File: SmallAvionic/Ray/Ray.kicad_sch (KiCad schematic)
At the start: 12 parts, among them U1 STM32F103C8Tx, U2 BMI088

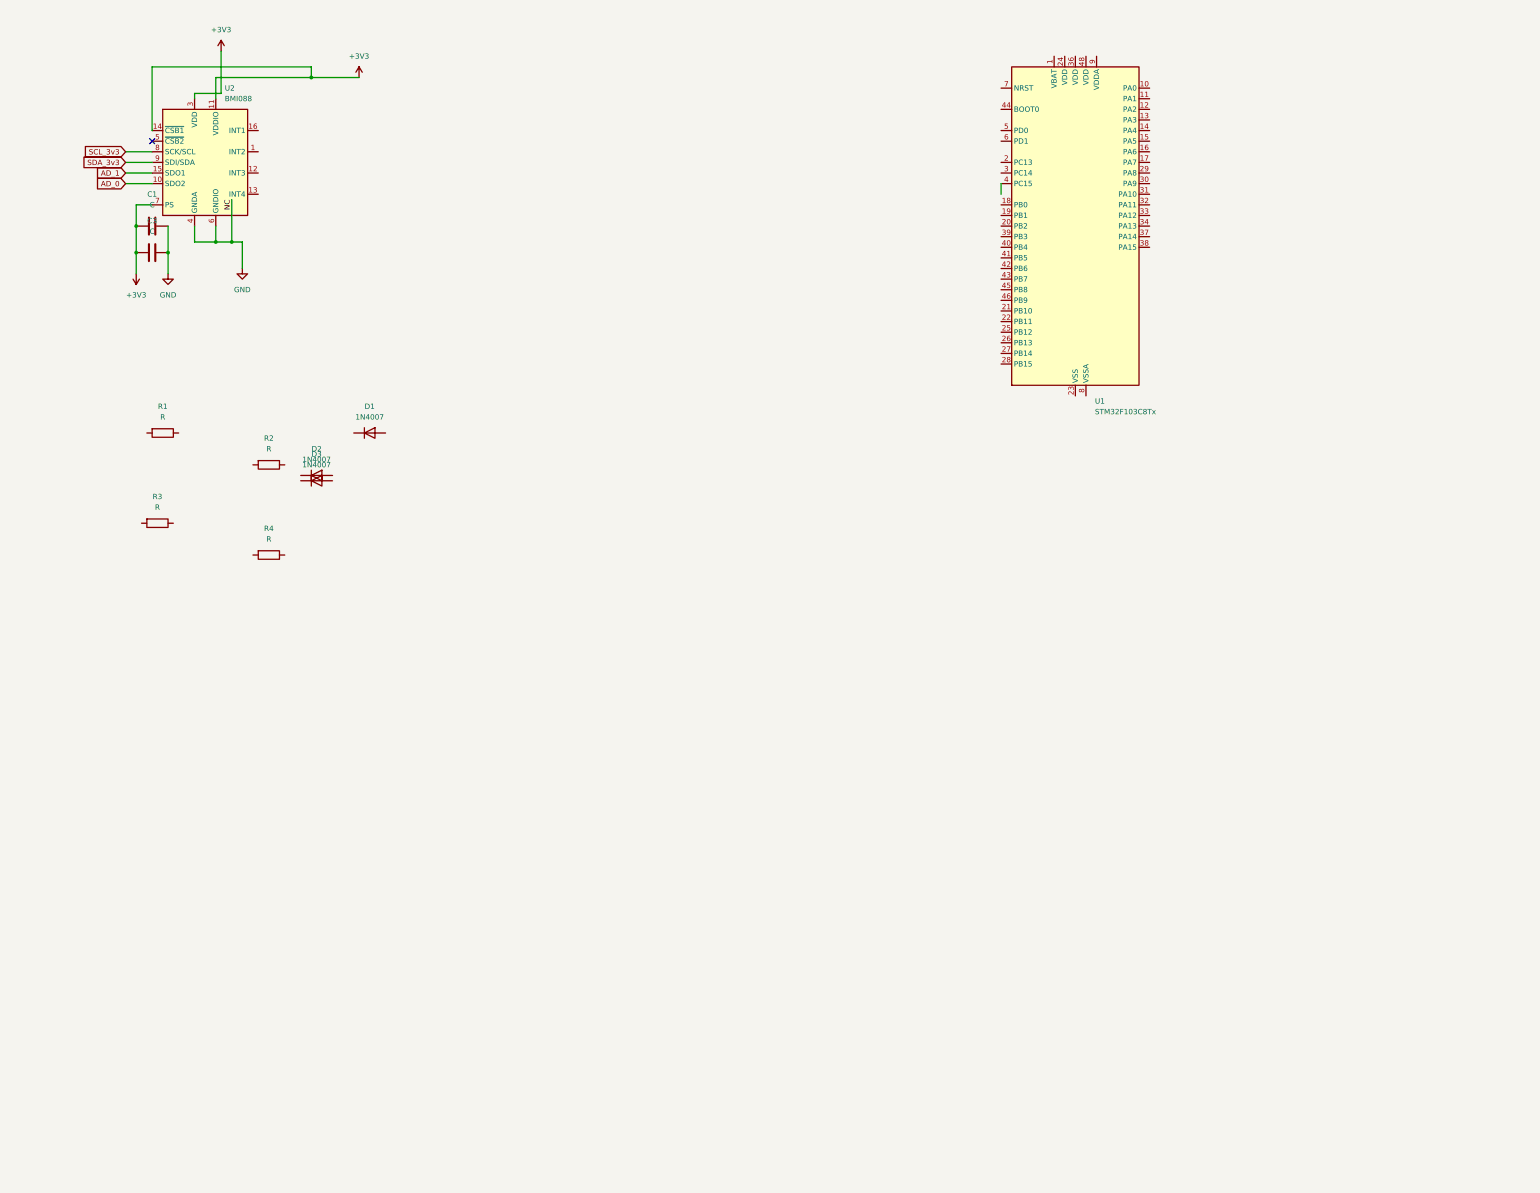
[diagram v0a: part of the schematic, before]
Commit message: Ray finish IMU,BMP, Madnetometer. But just whatever3 7 21 copy from internet
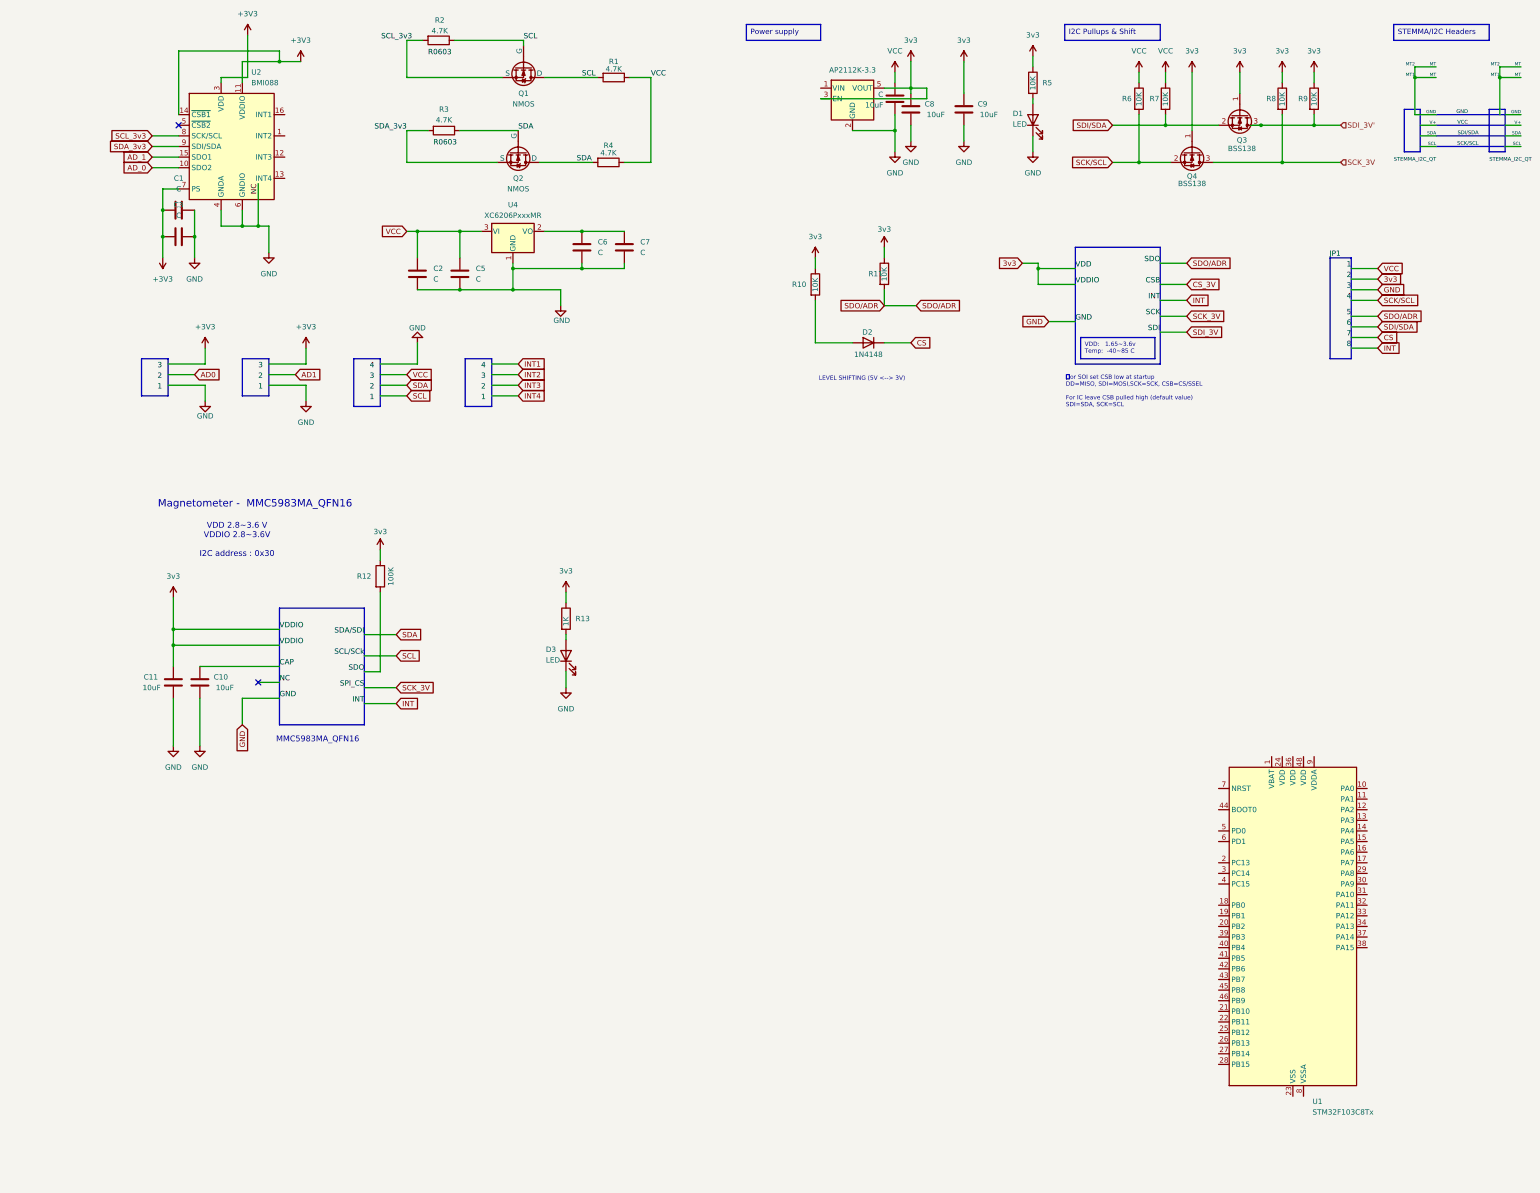
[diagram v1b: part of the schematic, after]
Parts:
- removed D1, D2, D3: 1N4007, Diode_THT:D_DO-41_SOD81_P10.16mm_Horizontal, symbol Diode:1N4007
- added C, C10, C11, C8, C9: 10uF, symbol Device:C
- added C2, C5, C6, C7: C, symbol Device:C
- added D1, D3: LED, symbol Device:LED
- added D2: 1N4148, Diode_THT:D_DO-35_SOD27_P7.62mm_Horizontal, symbol Diode:1N4148
- added Q1, Q2: NMOS, symbol Simulation_SPICE:NMOS
- added Q3, Q4: BSS138, Package_TO_SOT_SMD:SOT-23, symbol Transistor_FET:BSS138
- added R10, R11, R5, R6, R7, R8, R9: 10K, symbol Device:R
- added R12: 100K, symbol Device:R
- added R13: 1K, symbol Device:R
- added U3: AP2112K-3.3, Package_TO_SOT_SMD:SOT-23-5, symbol Regulator_Linear:AP2112K-3.3
- added U4: XC6206PxxxMR, Package_TO_SOT_SMD:SOT-23-3, symbol Regulator_Linear:XC6206PxxxMR
- R1: renamed from R2; value R -> 4.7K
- R2: renamed from R1; value R -> 4.7K
- R3, R4: value R -> 4.7K
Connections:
- net GND: now also C.2, C10.2, C11.2, C2.2, C5.2, C6.2, C7.2, C8.2, C9.2, D1.1 (K), D3.1 (K), U3.2 (GND), U4.1 (GND)
- net SCL_3v3: now also R2.2, Q1.3 (S)
- net SDA_3v3: now also R3.2, Q2.3 (S)
- net VCC: now reaches R4.1
- net VCC: now also R1.1, C.1, C2.1, C5.1, R6.1, R7.1, U4.3 (VI)
- net SDA: now reaches R4.2
- net SDA: now also R3.1, Q2.1 (D), Q2.2 (G)
- net SCL: now reaches R1.2
- net SCL: now also R2.1, Q1.1 (D), Q1.2 (G)
- new net: C6.1, C7.1, U4.2 (VO)
- new net: D2.2 (A), R10.2
- new net: D3.2 (A), R13.2
- new net: D1.2 (A), R5.2
- new net 3v3: C11.1, C8.1, C9.1, Q3.1 (G), Q4.1 (G), R10.1, R11.1, R12.1, R13.1, R5.1, R8.1, R9.1, U3.3 (EN), U3.5 (VOUT)
- new net CAP: C10.1
- new net CS: D2.1 (K)
- new net SCK_3V: Q4.3 (D), R8.2
- new net SCK/SCL: Q4.2 (S), R6.2
- new net SDI_3V': Q3.3 (D), R9.2
- new net SDI/SDA: Q3.2 (S), R7.2
- new net SDO/ADR: R11.2, R12.2
- no-connect marks 1 -> 2
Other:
- note added: "LEVEL SHIFTING (5V <--> 3V)"
- note added: "MMC5983MA_QFN16"
- note added: "Magnetometer - MMC5983MA_QFN16"
- note added: "VDD 2.8~3.6 V VDDIO 2.8~3.6V I2C address : 0x30"
- note added: "Ｆor SOI set CSB low at startup DD=MISO, SDI=MOSI,SCK=SCK, CSB=CS/SSEL For IC leave CSB pulled high (default value) SDI=SDA, SCK=SCL"
- moved on the sheet: C1, C3, R1, R2, R3, R4, U1, U2
